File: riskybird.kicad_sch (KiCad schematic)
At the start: 83 parts, among them J1 USB_B_Micro, J2 Conn_01x02, J3 Conn_01x02, J4 Conn_01x02, J5 Conn_01x02, J6 Conn_01x02, J7 Conn_01x10, J8 Conn_01x10, Q1 SI2302, Q2 SI2302, Q3 SI2302, Q4 SI2302, Q5 DNBT8105-7, Q6 DNBT8105-7, Q7 Q_NMOS_GSD, SW1 SW_SPST, SW2 SW_SPST, SW3 SW_SPST, U1 MCP73831-2-OT, U3 TPS2113A, U4 LP2985-3.0, U6 ESP32-C3-WROOM-02, U7 BMI088, U8 FT231XS

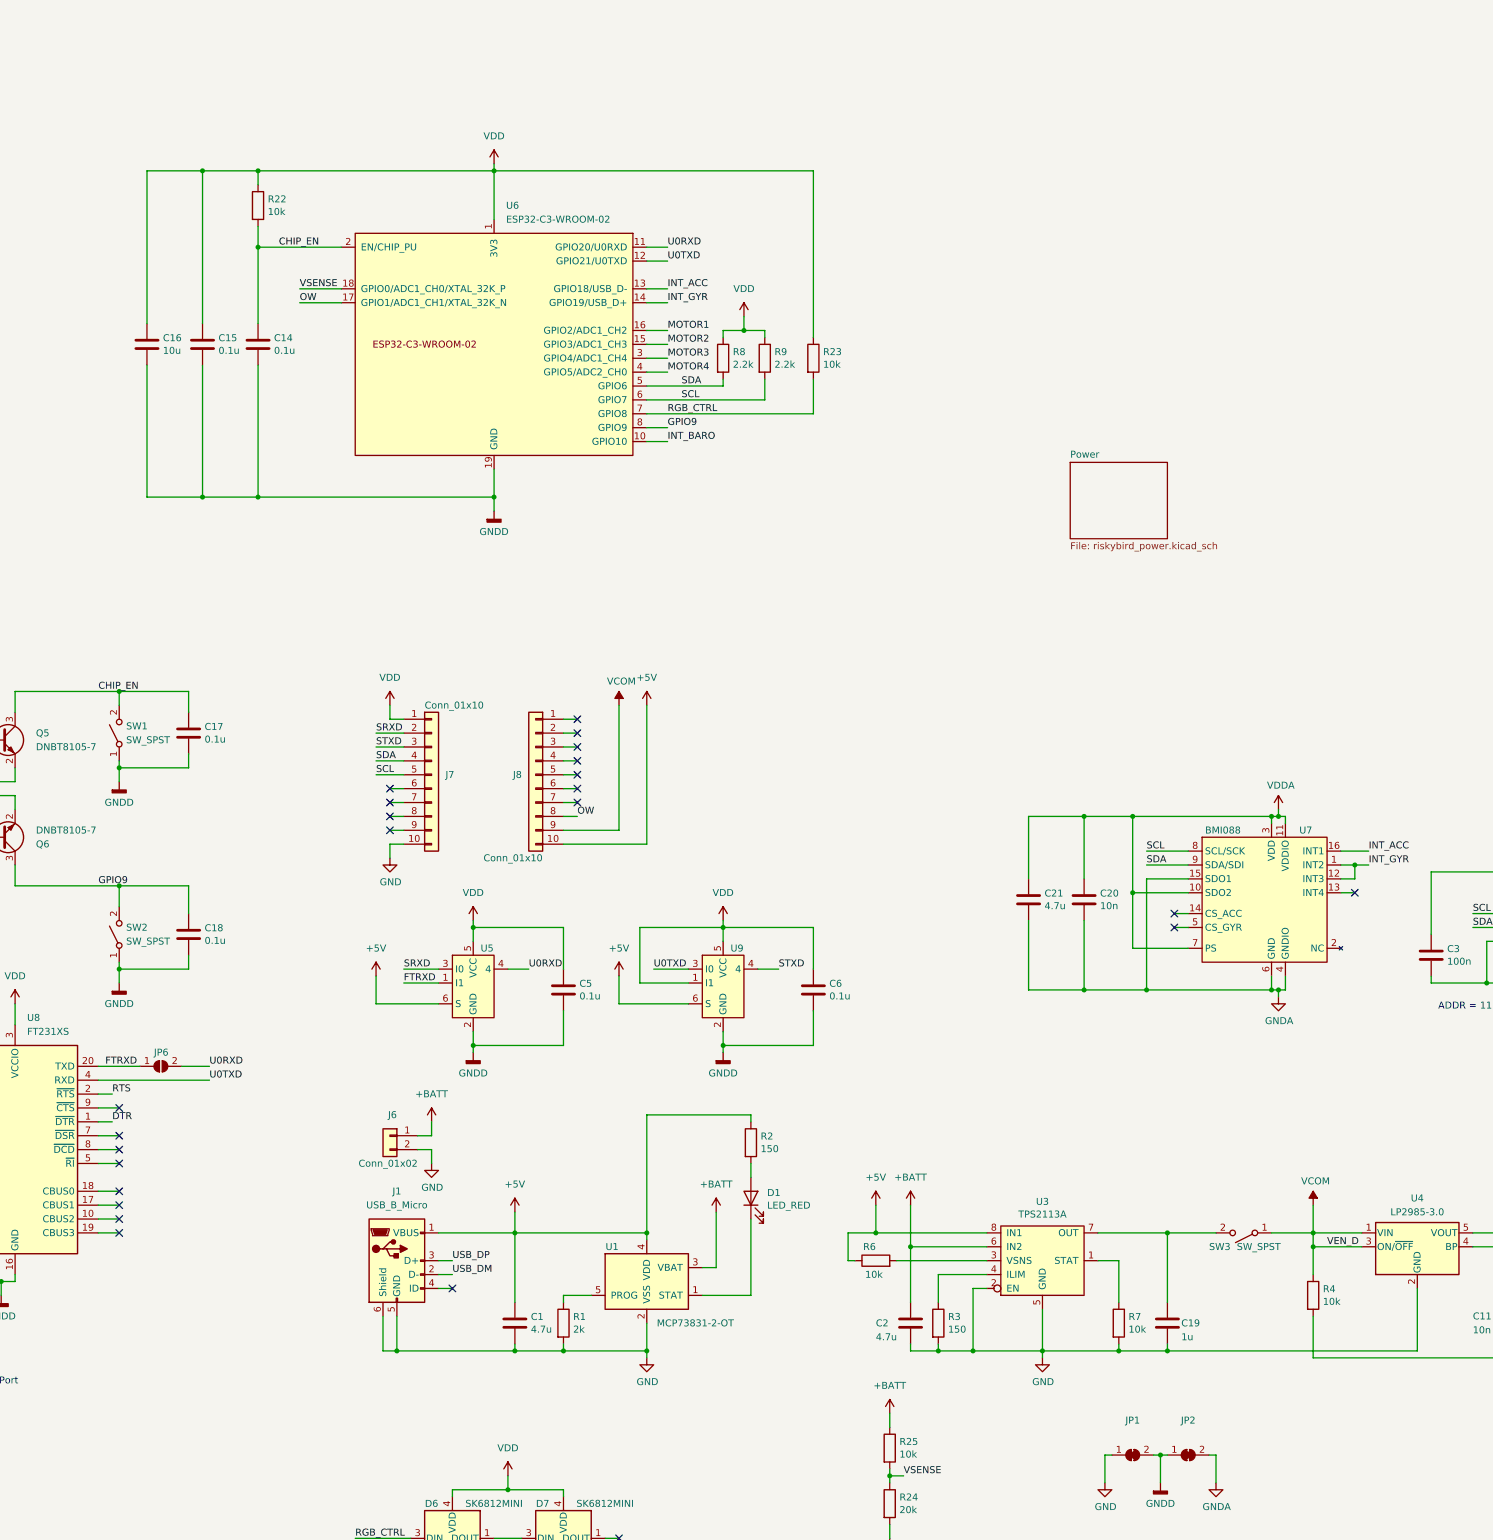
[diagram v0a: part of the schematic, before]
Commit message: finish routing
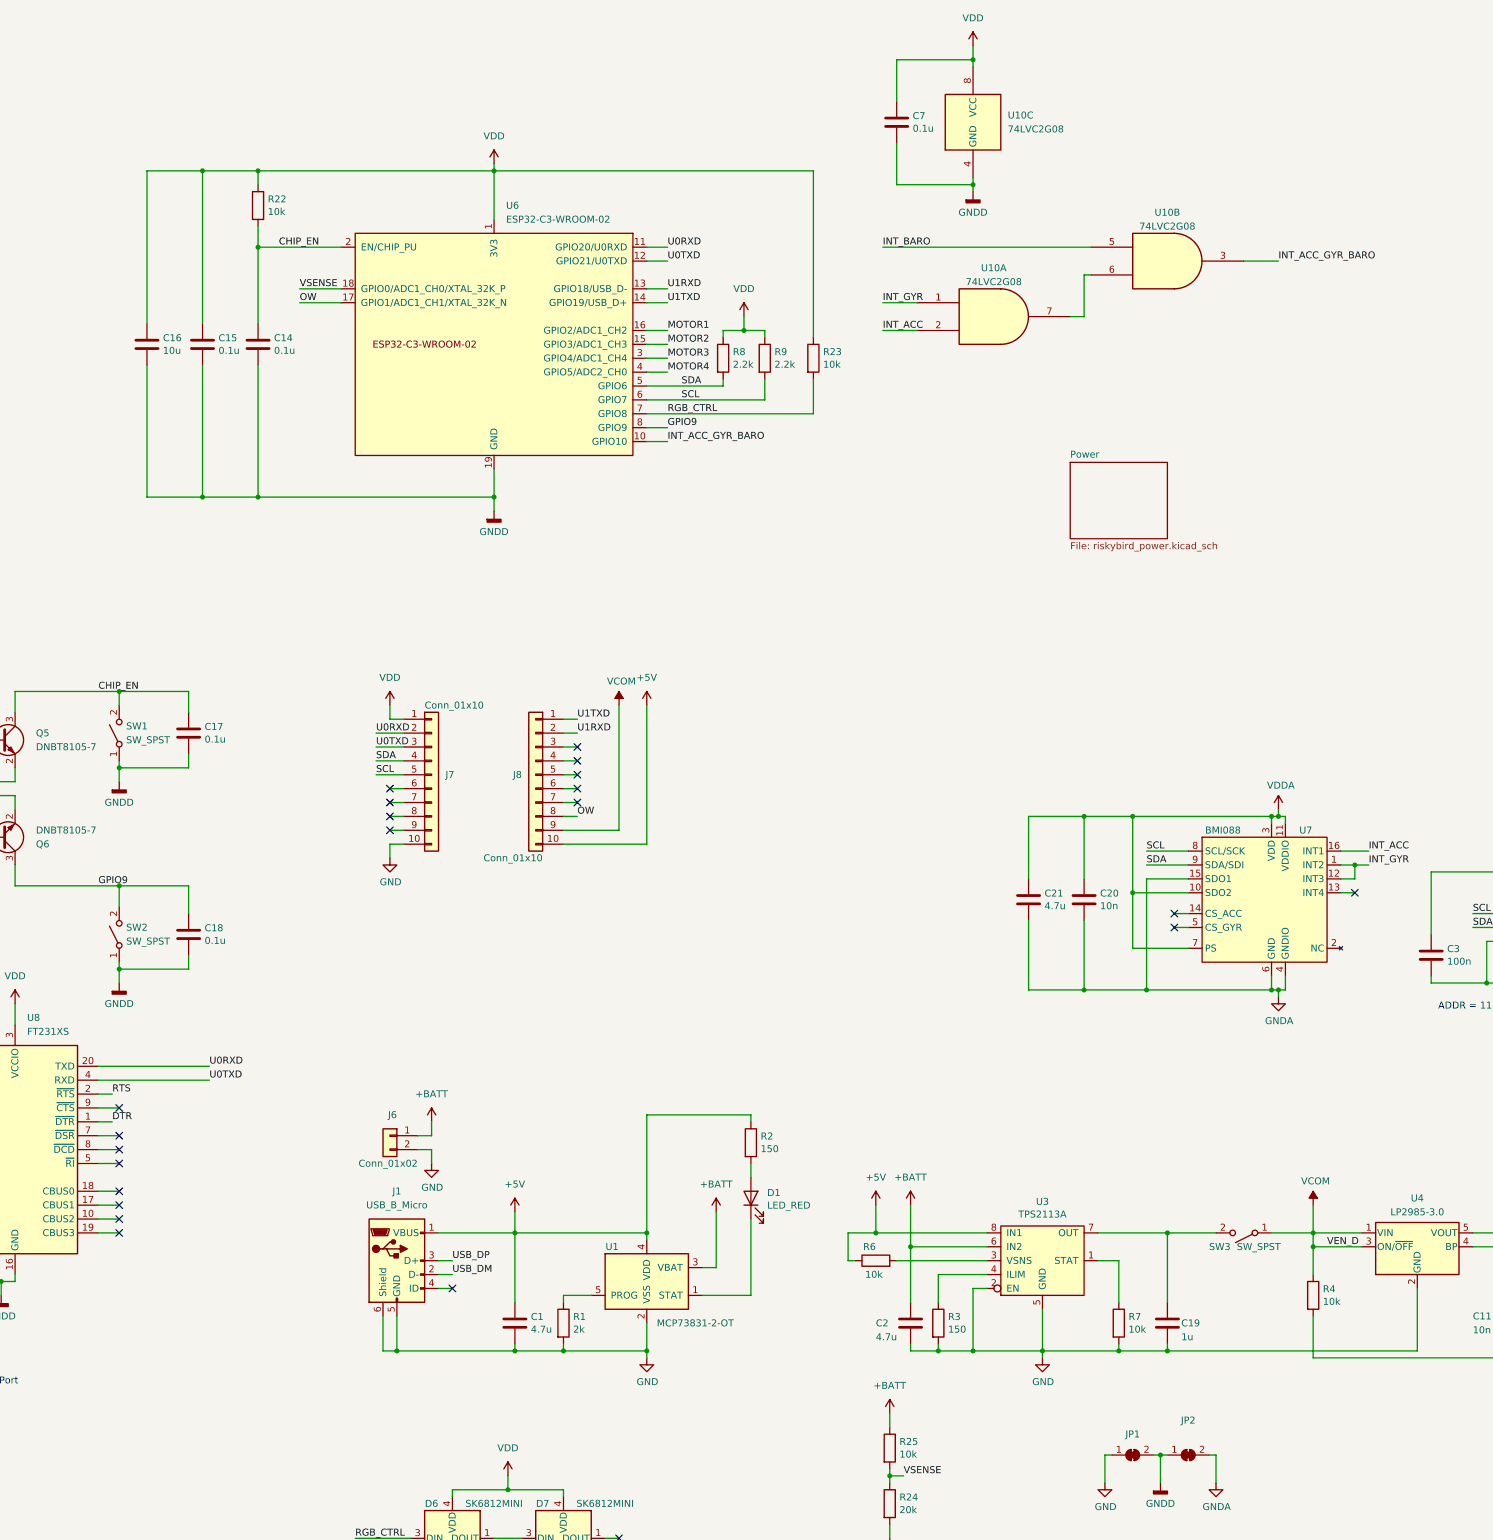
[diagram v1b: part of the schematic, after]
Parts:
- removed C5, C6: 0.1u, Capacitor_SMD:C_0603_1608Metric_Pad1.08x0.95mm_HandSolder, symbol Device:C
- removed JP6: SolderJumper_2_Bridged, Jumper:SolderJumper-2_P1.3mm_Open_Pad1.0x1.5mm, symbol Jumper:SolderJumper_2_Open
- removed U5, U9: ~, Package_TO_SOT_SMD:SOT-363_SC-70-6, symbol riskybird:74LVC1G157
- added C7: 0.1u, Capacitor_SMD:C_0603_1608Metric_Pad1.08x0.95mm_HandSolder, symbol Device:C
- added U10: 74LVC2G08, Package_SO:VSSOP-8_3.0x3.0mm_P0.65mm, symbol 74xGxx:74LVC2G08
- JP1, JP2: footprint Jumper:SolderJumper-2_P1.3mm_Bridged_Pad1.0x1.5mm -> riskybird:shunt
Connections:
- net FTRXD is gone; now on net U0RXD: U8.20 (TXD)
- net SRXD is gone; now on net U0RXD: J7.2 (Pin_2)
- net STXD is gone; now on net U0TXD: J7.3 (Pin_3)
- net GNDD: now also C7.2, U10.4 (GND)
- net INT_ACC: now also U10.2; no longer U6.13 (GPIO18/USB_D-)
- net INT_BARO: now also U10.5; no longer U6.10 (GPIO10)
- net INT_GYR: now also U10.1; no longer U6.14 (GPIO19/USB_D+)
- net VDD: now also C7.1, U10.8 (VCC)
- net U1TXD: now reaches J8.1 (Pin_1)
- net U1TXD: now also U6.14 (GPIO19/USB_D+)
- net U1RXD: now reaches J8.2 (Pin_2)
- net U1RXD: now also U6.13 (GPIO18/USB_D-)
- new net: U10.6, U10.7
- new net INT_ACC_GYR_BARO: U10.3, U6.10 (GPIO10)
- no-connect marks 25 -> 23
